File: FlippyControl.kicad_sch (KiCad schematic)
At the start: 24 parts, among them J1 WiiNunchuck, J2 WiiNunchuck, J3 Data Harness Out, J4 USB_C_Receptacle_USB2.0, P1 Power, P2 Analog, P3 Digital, P4 Digital, P5 CONN_01X01, P6 CONN_01X01, P7 CONN_01X01, P8 CONN_01X01, U1 mini_esp32

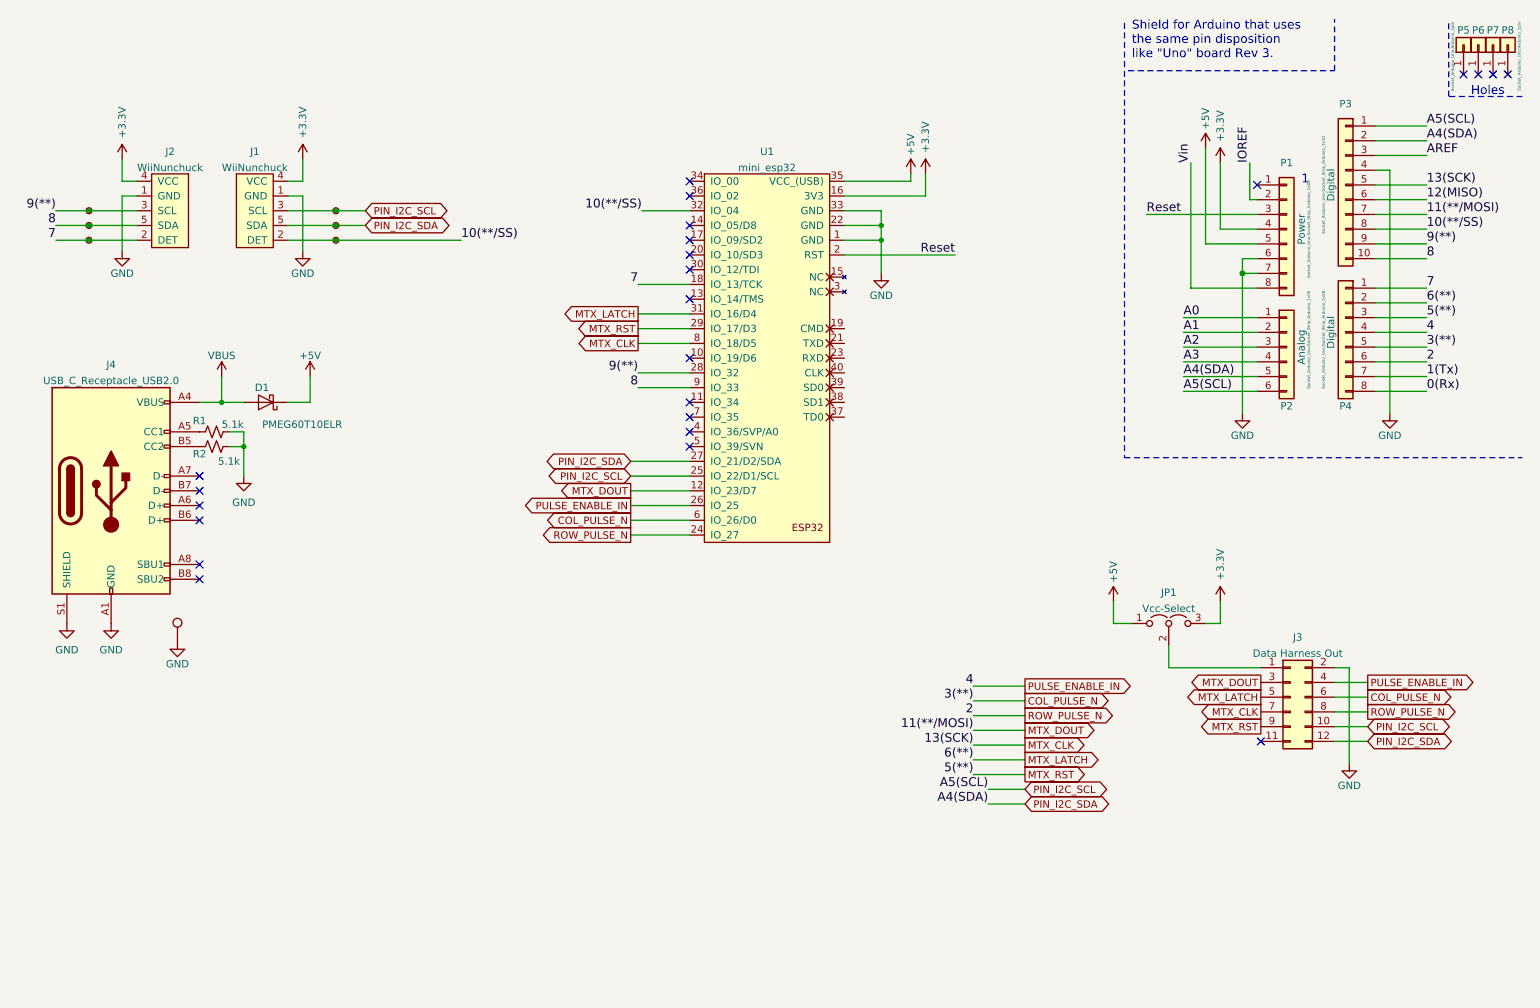
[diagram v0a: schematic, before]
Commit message: Add submodule and migrate project
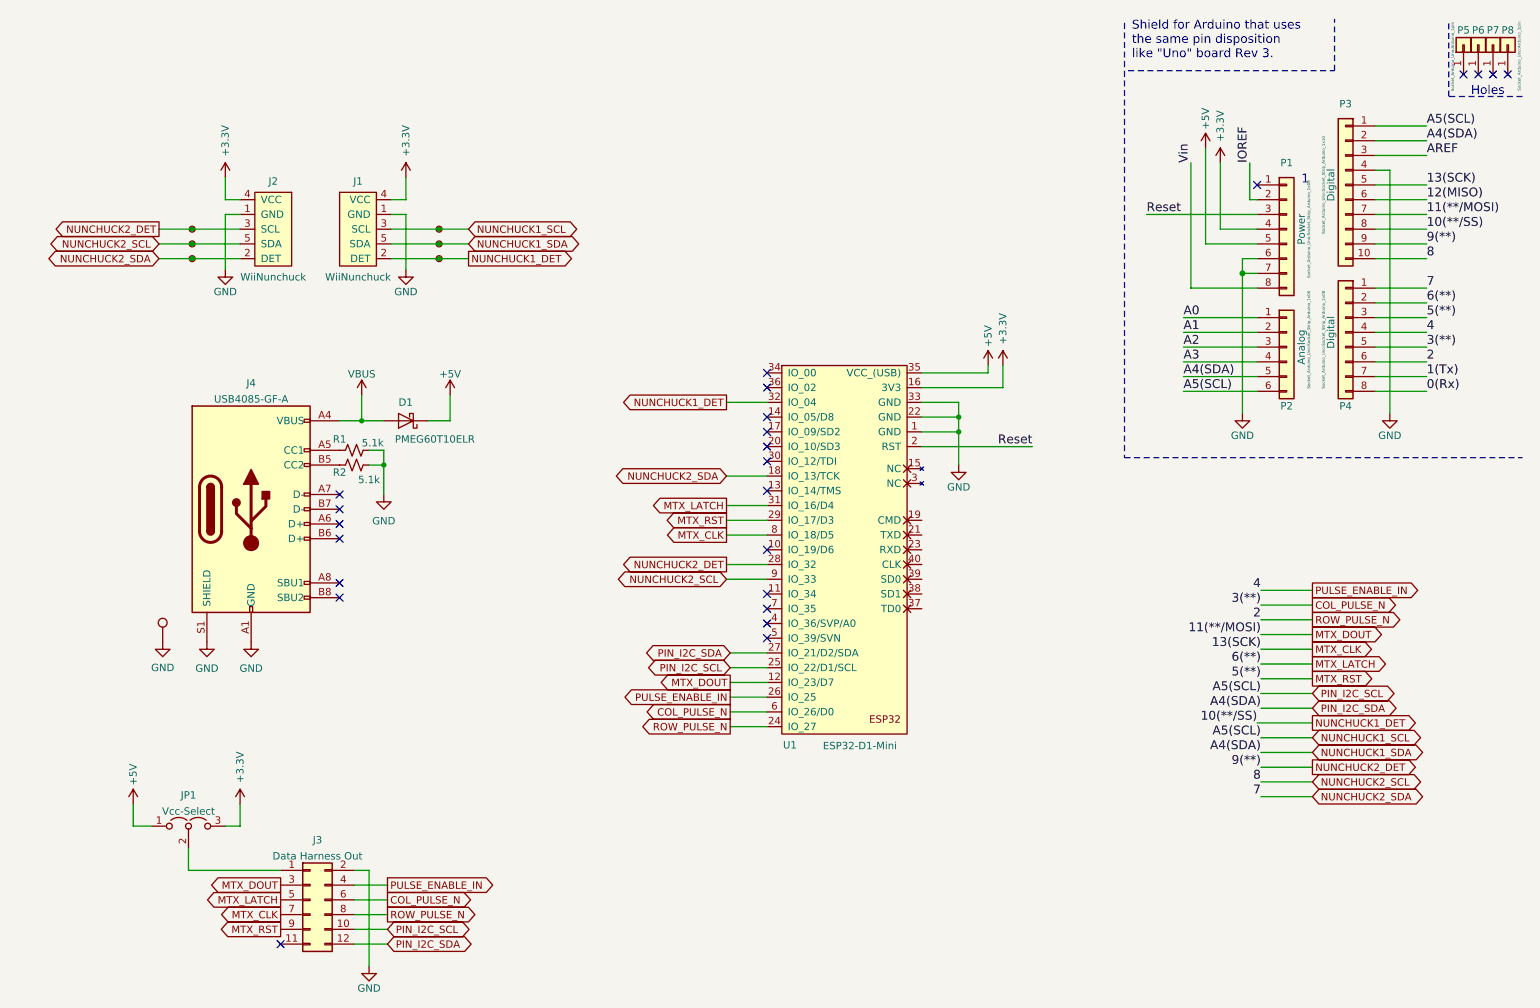
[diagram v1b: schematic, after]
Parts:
- D1: footprint Diode_SMD:Nexperia_CFP3_SOD-123W -> Diode_SMD:D_SOD-123
- J1, J2: footprint FlippyControl:WiiNunchuck -> Nieto_Connector:WiiNunchuck; symbol FlippyControl:WiiNunchuck -> Nieto_Connector:WiiNunchuck; now left out of the parts list
- J4: value USB_C_Receptacle_USB2.0 -> USB4085-GF-A
- U1: value mini_esp32 -> ESP32-D1-Mini; footprint FlippyControl:ESP32_mini -> Nieto_Module:ESP32_mini; symbol FlippyControl:mini_esp32 -> Nieto_MCU_Espressif:ESP32-D1-Mini
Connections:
- net 10(**/SS) renamed NUNCHUCK1_DET
- net 7 renamed NUNCHUCK2_SDA
- net 8 renamed NUNCHUCK2_SCL
- net 9(**) renamed NUNCHUCK2_DET
- net PIN_I2C_SCL renamed NUNCHUCK1_SCL
- net PIN_I2C_SDA renamed NUNCHUCK1_SDA
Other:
- moved on the sheet: D1, J1, J2, J3, J4, JP1, R1, R2, U1

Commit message: Final Rev.B, adding RasPi connector and PWM output
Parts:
- removed P6, P8: CONN_01X01, Socket_Arduino_Uno:Arduino_1pin, symbol Connector_Generic:Conn_01x01
- removed TP1: CTL2_SCL, TestPoint:TestPoint_Pad_D3.0mm, symbol Connector:TestPoint_Small
- removed TP2: CTL1_SCL, TestPoint:TestPoint_Pad_D3.0mm, symbol Connector:TestPoint_Small
- removed TP3: CTL2_SDA, TestPoint:TestPoint_Pad_D3.0mm, symbol Connector:TestPoint_Small
- removed TP4: CTL1_SDA, TestPoint:TestPoint_Pad_D3.0mm, symbol Connector:TestPoint_Small
- removed TP5: CTL2_DET, TestPoint:TestPoint_Pad_D3.0mm, symbol Connector:TestPoint_Small
- removed TP6: CTL1_DET, TestPoint:TestPoint_Pad_D3.0mm, symbol Connector:TestPoint_Small
- added J5: RasPI-40Pin, Connector_IDC:IDC-Header_2x20_P2.54mm_Vertical, symbol raspberrypi_hat:OX40HAT
- added J6: WP, Connector_PinHeader_2.54mm:PinHeader_1x02_P2.54mm_Vertical, symbol Connector_Generic:Conn_01x02
- added JP2: 5V_RET, Connector_PinHeader_2.54mm:PinHeader_1x02_P2.54mm_Vertical, symbol Jumper:Jumper_2_Open
- added R3: DNP, Resistor_SMD:R_0603_1608Metric, symbol Device:R
- added R4: 10K, Resistor_SMD:R_0603_1608Metric, symbol Device:R
- added R5, R6: 3.9k, Resistor_SMD:R_0603_1608Metric, symbol Device:R
- added SW1: RESET, Button_Switch_SMD:SW_SPST_PTS645, symbol Switch:SW_Push
- added U2: CAT24C32, Package_SO:SOIC-8_3.9x4.9mm_P1.27mm, symbol raspberrypi_hat:CAT24C32
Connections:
- net A3 is gone; now on net NUNCHUCK2_DET: P2.4 (Pin_4)
- net +3V3: now also J5.1 (P3V3), J5.17 (P3V3), R4.1, R5.1, R6.1, U2.8 (VCC)
- net +5V: now also J5.2 (P5V), J5.4 (P5V)
- net GND: now also J3.12 (Pin_12), J5.14 (GND), J5.20 (GND), J5.25 (GND), J5.30 (GND), J5.34 (GND), J5.39 (GND), J5.6 (GND), J5.9 (GND), J6.1 (Pin_1), R3.2, SW1.1, U2.1 (A0), U2.2 (A1), U2.3 (A2), U2.4 (GND)
- net NUNCHUCK1_SCL: no longer J3.10 (Pin_10)
- net NUNCHUCK1_SDA: no longer J3.12 (Pin_12)
- net NUNCHUCK2_DET: no longer P3.9 (Pin_9)
- net Reset: now also SW1.2
- net VBUS: now also JP2.2 (B)
- net MAX3000_AUX_5V: now reaches J3.11 (Pin_11)
- net MAX3000_AUX_5V: now also JP2.1 (A)
- net MAX3000_LED_PWM: now reaches U1.30 (IO_12/TDI)
- net MAX3000_LED_PWM: now also J3.10 (Pin_10), P3.9 (Pin_9), J5.33 (BCM13)
- net COL_PULSE_N renamed MAX3000_COL
- net MAX3000_COL: now also J5.37 (BCM26)
- net MTX_CLK renamed MAX3000_SCK
- net MAX3000_SCK: now also J5.23 (BCM11)
- net MTX_DOUT renamed MAX3000_MOSI
- net MAX3000_MOSI: now also J5.19 (BCM10)
- net MTX_LATCH renamed MAX3000_LATCH
- net MAX3000_LATCH: now also J5.11 (BCM17)
- net MTX_RST renamed MAX3000_RST
- net MAX3000_RST: now also J5.13 (BCM27)
- net PULSE_ENABLE_IN renamed MAX3000_PULSE
- net MAX3000_PULSE: now also J5.15 (BCM22)
- net ROW_PULSE_N renamed MAX3000_ROW
- net MAX3000_ROW: now also J5.29 (BCM5)
- new net: J6.2 (Pin_2), R3.1, R4.2, U2.7 (WP)
- new net EEPROM_SCL: J5.28 (BCM1), R5.2, U2.6 (SCL)
- new net EEPROM_SDA: J5.27 (BCM0), R6.2, U2.5 (SDA)
- new net MAX3000_SCL: J5.5 (BCM3)
- new net MAX3000_SDA: J5.3 (BCM2)
- no-connect marks 24 -> 36
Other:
- moved on the sheet: D1, J1, J2, J3, J4, JP1, P1, P2, P3, P4, P5, P7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

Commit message: Add pullups, fix miswired pads
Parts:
- added R10, R11, R12, R7, R8, R9: 4.7k, Resistor_SMD:R_0603_1608Metric, symbol Device:R_Small_US
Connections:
- net +3V3: now also R10.2, R11.2, R12.2, R7.2, R8.2, R9.2
- net MAX3000_LED_PWM: now also J5.12 (BCM18); no longer J5.33 (BCM13)
- net NUNCHUCK1_DET: now also R9.1
- net NUNCHUCK1_SCL: now also R7.1
- net NUNCHUCK1_SDA: now also R8.1
- net NUNCHUCK2_DET: now also J2.2 (DET), R12.1; no longer J2.3 (SCL)
- net NUNCHUCK2_SCL: now also J2.3 (SCL), R10.1; no longer J2.5 (SDA)
- net NUNCHUCK2_SDA: now also J2.5 (SDA), R11.1; no longer J2.2 (DET)
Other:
- note added: "All components optional. Footprints are included to match Hat specifications."
- note added: "Arduino Header"
- note added: "Aux 5V is only present on Revision D and higher of driver boards"
- note added: "ESP32 Header"
- note added: "Only populate pull-down resistors and protection diode if USB-C in use."
- note added: "Only populate pull-up resistors if Wiimotes in use."
- note added: "Raspberry Pi Hat EEPROM"
- note added: "Raspberry Pi Header"
- note added: "USB-C Power Input"
- note added: "Wiimote Connectors"
- note removed: "Shield for Arduino that uses the same pin disposition like "Uno" board Rev 3."
- moved on the sheet: D1, J1, J2, J3, J4, J5, J6, JP1, JP2, P1, P2, P3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
